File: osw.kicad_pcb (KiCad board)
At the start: 2 copper layers, 46 x 41.4 mm, 60 parts, among them J1 Conn_01x02, J2 microSD_MEM2067-02-180-00-A_R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, J3 2169890001, Q1 Q_NMOS_ToshibaSMD, SW1 SPST_EVQ-P7J01P, SW2 SPST_EVQ-P7J01P, SW3 SPST_EVQ-P7J01P, SW4 SPST_EVQ-P7J01P, U1 L96-M33, U10 BMA400, U11 GC9A01_IPS_display_SPI, U12 esd_USB_IP4234CZ6, U13 BH1792GLC-E2, U2 TPS22933, U3 ESP32-MINI-1, U4 MCP73831T-2ACI, U5 MIC5504-3p3, U6 FT234XD-R, U7 MIC5504-3p3, U8 23K256-I/SN, U9 PCF85063ATL/1,118

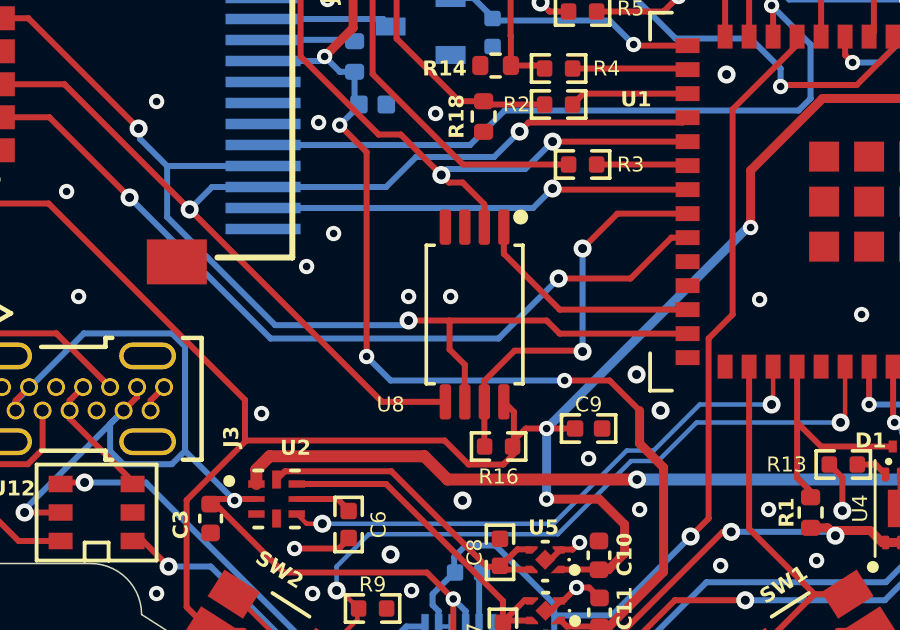
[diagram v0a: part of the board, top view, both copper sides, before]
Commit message: Updates.
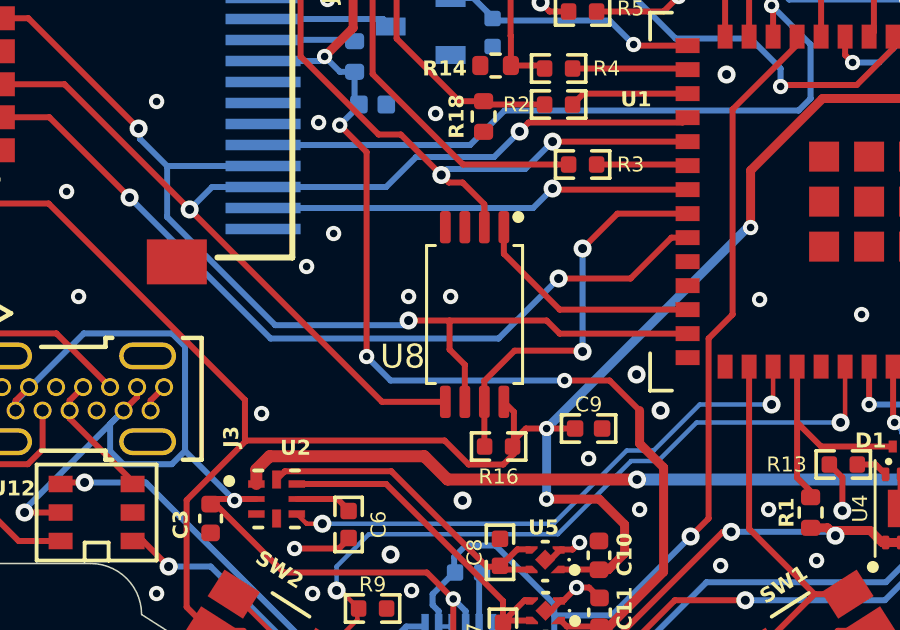
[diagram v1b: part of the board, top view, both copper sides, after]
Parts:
- U8: footprint AllardSOP:SOP8P65_300X640X120L47X24N -> AllardSOP:SOP8P65_300X640X120L47X24L
